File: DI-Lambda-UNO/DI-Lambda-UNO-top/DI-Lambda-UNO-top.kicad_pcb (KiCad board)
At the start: 2 copper layers, 38.2 x 125 mm, 4 parts, among them J1 CONN_02X04, J2 CONN_02X04, J3 CONN_02X04, J4 CONN_02X04

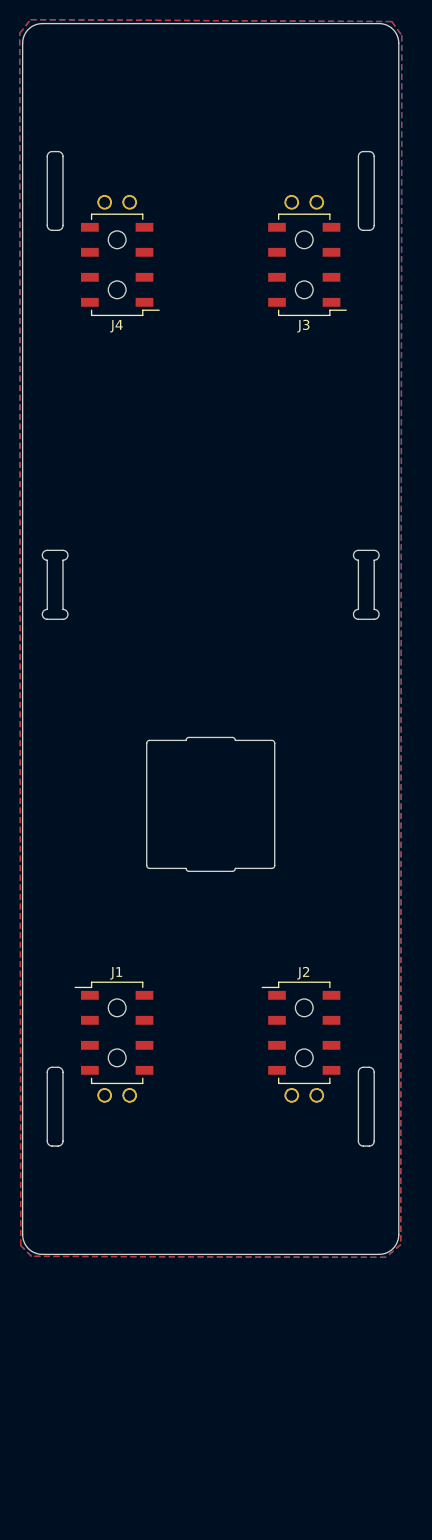
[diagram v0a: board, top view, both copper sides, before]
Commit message: Version 1.5
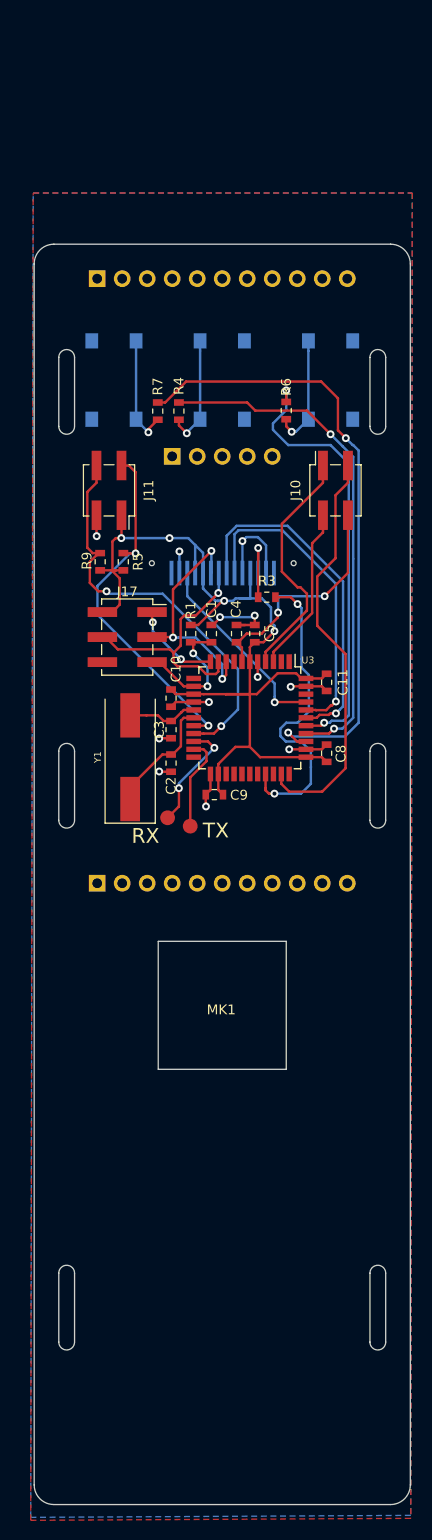
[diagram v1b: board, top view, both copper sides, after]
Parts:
- added C1: 0.1uF 25v, Capacitor_SMD:C_0603_1608Metric, F.Cu at (149.3, 80.7)
- added C10: 0.1uF 25v, Capacitor_SMD:C_0603_1608Metric, F.Cu at (145.2, 87.3)
- added C11: 0.1uF 25v, Capacitor_SMD:C_0603_1608Metric, F.Cu at (161.0, 85.7)
- added C2: 22pF 25V, Capacitor_SMD:C_0603_1608Metric, F.Cu at (145.2, 93.9)
- added C3: 22pF 25V, Capacitor_SMD:C_0603_1608Metric, F.Cu at (145.2, 90.5)
- added C4: 4.7uF 25V, Capacitor_SMD:C_0603_1608Metric, F.Cu at (151.8, 80.7)
- added C5: 1uF 25V, Capacitor_SMD:C_0603_1608Metric, F.Cu at (153.7, 80.7)
- added C8: 0.1uF 25v, Capacitor_SMD:C_0603_1608Metric, F.Cu at (161.0, 92.9)
- added C9: 0.1uF 25v, Capacitor_SMD:C_0603_1608Metric, F.Cu at (149.6, 97.1)
- added J10: Conn_02x02_Odd_Even, Connector_PinSocket_2.54mm:PinSocket_2x02_P2.54mm_Vertical_SMD, F.Cu at (161.9, 66.2)
- added J11: Conn_02x02_Odd_Even, Connector_PinSocket_2.54mm:PinSocket_2x02_P2.54mm_Vertical_SMD, F.Cu at (138.9, 66.2)
- added J12: Conn_01x05, Connector_PinHeader_2.54mm:PinHeader_1x05_P2.54mm_Vertical, B.Cu at (145.3, 62.7)
- added J13: Conn_01x11, Connector_PinHeader_2.54mm:PinHeader_1x11_P2.54mm_Vertical, B.Cu at (137.7, 106.1)
- added J17: CONN_02X03, Connector_PinSocket_2.54mm:PinSocket_2x03_P2.54mm_Vertical_SMD, F.Cu at (140.7, 81.1)
- added J5: Conn_01x11, Connector_PinHeader_2.54mm:PinHeader_1x11_P2.54mm_Vertical, B.Cu at (137.7, 44.7)
- added J6: Conn_02x03_Odd_Even, Board_grooves:Pocket_1.6mm_7mm_no_cap, B.Cu at (166.2, 96.2)
- added J7: Conn_02x03_Odd_Even, Board_grooves:Pocket_1.6mm_7mm_no_cap, B.Cu at (134.6, 96.2)
- added J8: Conn_02x04_Odd_Even, Board_grooves:Pocket_1.6mm_7mm_no_cap, B.Cu at (134.6, 149.2)
- added J9: Conn_02x04_Odd_Even, Board_grooves:Pocket_1.6mm_7mm_no_cap, B.Cu at (166.2, 56.2)
- added MK1: Mounting_Hole, DI-Lambda-module-tabs:Cuvette-cutout-top, F.Cu at (150.4, 118.5)
- added R1: 4.7k, Resistor_SMD:R_0603_1608Metric, F.Cu at (147.2, 80.7)
- added R3: 220R, Resistor_SMD:R_0603_1608Metric, F.Cu at (154.9, 77.0)
- added R4: 220R, Resistor_SMD:R_0603_1608Metric, F.Cu at (146.0, 58.1)
- added R5: 4.7k, Resistor_SMD:R_0603_1608Metric, F.Cu at (140.3, 73.4)
- added R6: 220R, Resistor_SMD:R_0603_1608Metric, F.Cu at (156.9, 58.1)
- added R7: 220R, Resistor_SMD:R_0603_1608Metric, F.Cu at (143.8, 58.1)
- added R9: 4.7k, Resistor_SMD:R_0603_1608Metric, F.Cu at (138.0, 73.4)
- added SW2: SW_BLANK, Button_Switch_SMD:SW_SPST_PTS645, B.Cu at (150.4, 55.0)
- added SW3: SW_SAMPLE, Button_Switch_SMD:SW_SPST_PTS645, B.Cu at (161.4, 55.0)
- added SW4: SW_MODE, Button_Switch_SMD:SW_SPST_PTS645, B.Cu at (139.4, 55.0)
- added U1: LCD_1.44_ST7735, LCD:LCD_1.44_ST7735, B.Cu at (150.4, 74.6)
- added U3: ATMEGA32U4-MU, Housings_QFP:TQFP-44_10x10mm_Pitch0.8mm, F.Cu at (153.2, 89.3)
- added Y1: 8Mhz, Crystals:Crystal_SMD_HC49-SD, F.Cu at (141.0, 93.3)
- J1, J3: value CONN_02X04 -> Conn_02x04_Odd_Even; footprint Female_socket_pitch254_smt_through-board:Pin_Header_Straight_2x04_Pitch2.54mm_SMD_2THT -> Board_grooves:Pocket_1.6mm_7mm_no_cap; moved to B.Cu
- J2, J4: value CONN_02X04 -> Conn_01X01; footprint Female_socket_pitch254_smt_through-board:Pin_Header_Straight_2x04_Pitch2.54mm_SMD_2THT -> Measurement_Points:Measurement_Point_Round-SMD-Pad_Small
- moved J3 106.2 mm to (166.2, 149.2), turned to 270 degrees
- moved J1 65.3 mm to (134.6, 56.2), turned to 270 degrees
- moved J4 57.5 mm to (147.1, 100.3), turned to 0 degrees
- moved J2 25.9 mm to (144.8, 99.4)
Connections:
- J2 pad 1: Net-(J2-Pad1) -> /RX
- J4 pad 1: Net-(J4-Pad1) -> /TX
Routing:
- net /VCC: track 0.00 -> 98.0 mm, vias 0 -> 4
- net /MODE: track 0.00 -> 63.8 mm, vias 0 -> 2
- net /BLANK: track 0.00 -> 52.0 mm, vias 0 -> 2
- net /SAMPLE: track 0.00 -> 45.2 mm, vias 0 -> 2
- net /SDA: track 0.00 -> 43.1 mm, vias 0 -> 2
- net /LED_PWM: track 0.00 -> 42.1 mm
- net GND: track 0.00 -> 41.3 mm, vias 0 -> 12
- net /SCL: track 0.00 -> 36.9 mm, vias 0 -> 2
- net /LCD_A0: track 0.00 -> 35.3 mm, vias 0 -> 1
- net /LCD_LED: track 0.00 -> 32.2 mm, vias 0 -> 2
- net /LCD_RST: track 0.00 -> 32.0 mm, vias 0 -> 1
- net /MOSI: track 0.00 -> 25.7 mm, vias 0 -> 1
- net /DP: track 0.00 -> 24.6 mm
- net /SCK: track 0.00 -> 24.4 mm, vias 0 -> 3
- net /VBUS: track 0.00 -> 23.4 mm, vias 0 -> 2
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- added copper zone on B.Cu, net GND
- added copper zone on F.Cu, net GND
- removed copper zone on B.Cu, net (none)
- removed copper zone on F.Cu, net (none)
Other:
- board size 38.2 x 125 mm -> 38.2 x 128 mm
- board text added: "DI-Lambda UNO v1.5"
- board text added: "RX"
- board text added: "TX"
- board text removed: "DI-Lambda UNO v1.3"
